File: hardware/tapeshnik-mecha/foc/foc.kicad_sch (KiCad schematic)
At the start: 32 parts, among them J1 Conn_01x03, J2 Conn_01x03, J3 Conn_01x02, J4 Conn_01x07, J5 Conn_01x03, J6 Conn_01x03, U1 STSPIN233, U2 INA181A1IDBVR, U3 MT6701, U4 INA181A1IDBVR, U5 RP2040-Zero, U6 MT6701, U7 STSPIN233, U8 INA181A1IDBVR, U9 INA181A1IDBVR

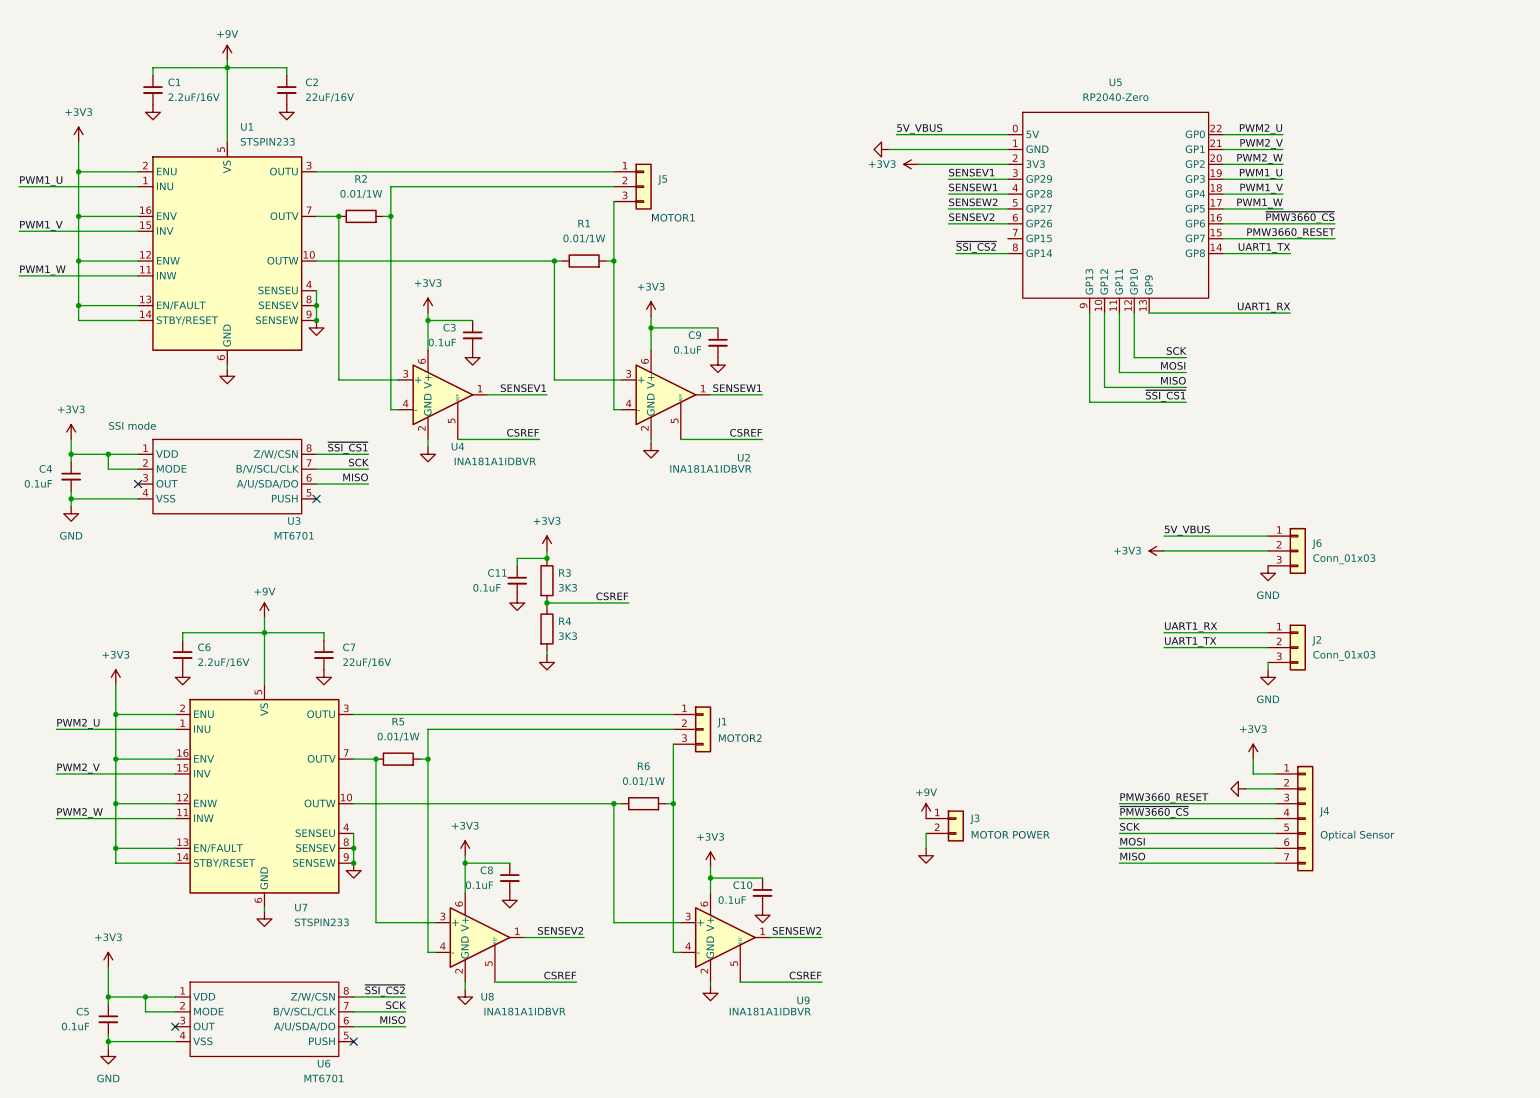
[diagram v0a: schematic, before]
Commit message: adding a lot of mecha-specific stuff
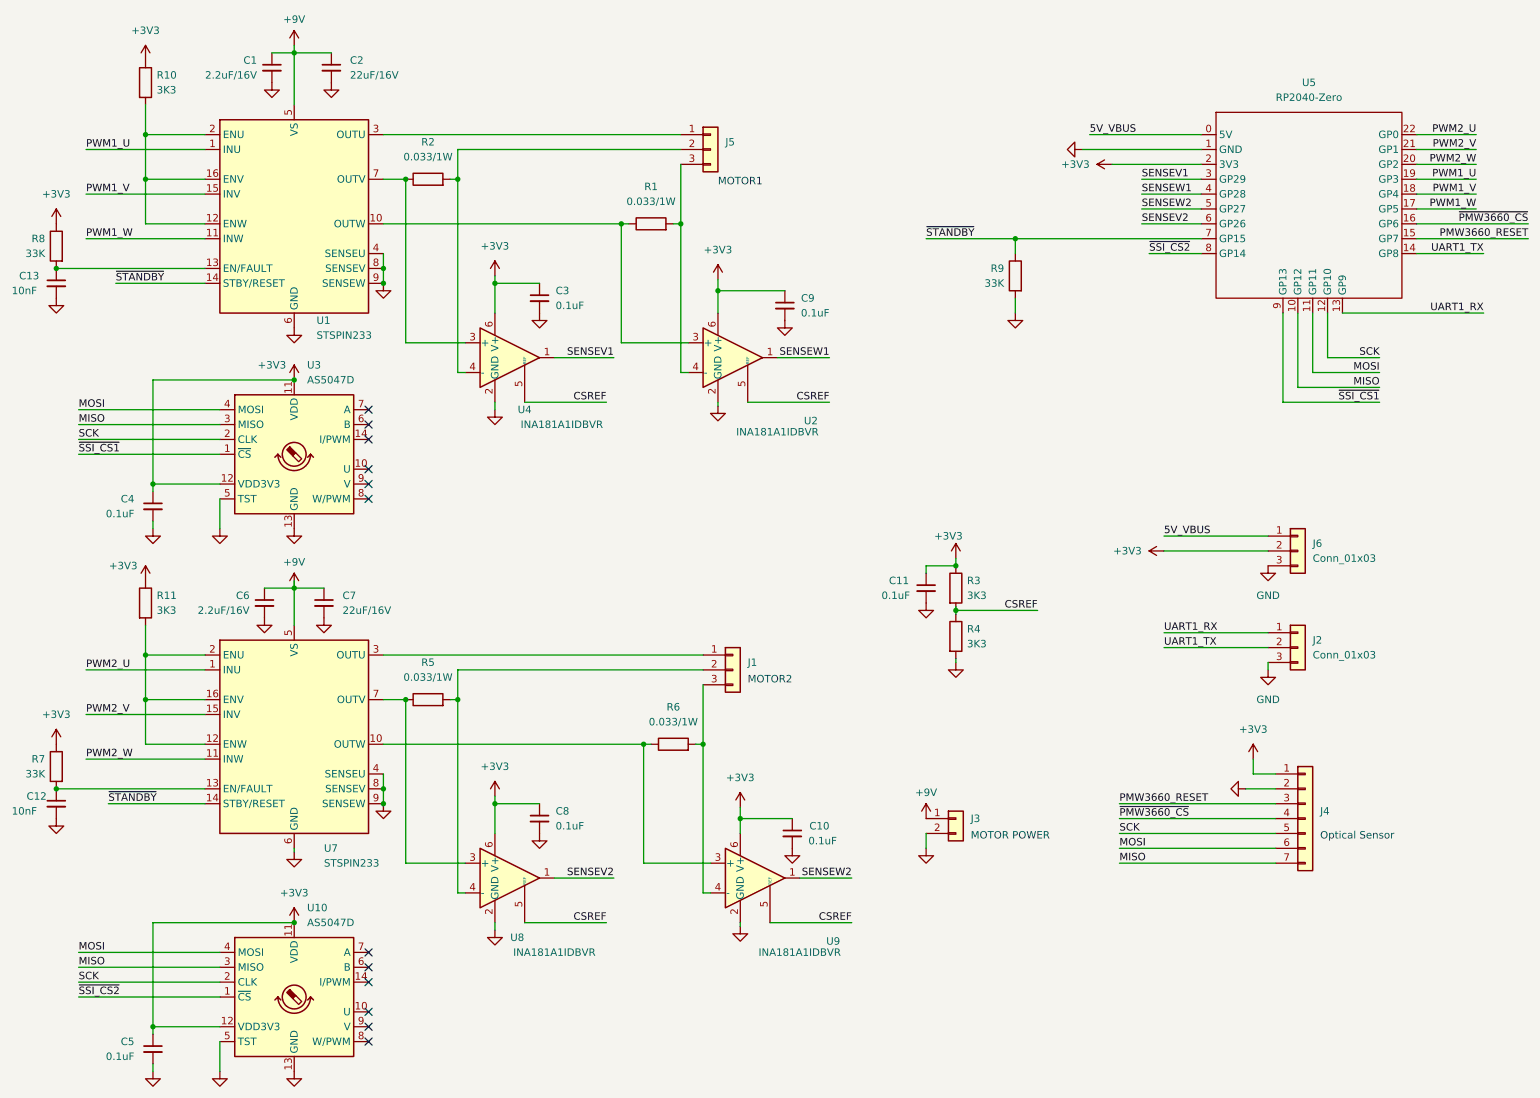
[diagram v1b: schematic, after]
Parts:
- removed U3, U6: MT6701, Package_SO:SOP-8_3.9x4.9mm_P1.27mm, symbol Magnetic_Encoder:MT6701
- added C12, C13: 10nF, Capacitor_SMD:C_0402_1005Metric, symbol Device:C_Small
- added R10, R11: 3K3, Resistor_SMD:R_0402_1005Metric, symbol Device:R
- added R7, R8: 33K, Resistor_SMD:R_0402_1005Metric, symbol Device:R
- added R9: 33K, Resistor_SMD:R_0603_1608Metric, symbol Device:R
- added U10, U3: AS5047D, Package_SO:TSSOP-14_4.4x5mm_P0.65mm, symbol Sensor_Magnetic:AS5047D
- C2, C7: footprint Capacitor_SMD:C_0603_1608Metric -> Capacitor_SMD:C_0805_2012Metric; LCSC (none) -> C45783
- R1, R2, R6: value 0.01/1W -> 0.033/1W; LCSC (none) -> C2934109
- R5: value 0.01/1W -> 0.033/1W; C55739 (none) -> C2934109
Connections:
- net +3V3: now also R10.1, R11.1, R7.1, R8.1, U10.11 (VDD), U10.12 (VDD3V3), U3.11 (VDD), U3.12 (VDD3V3); no longer U1.12 (ENW), U1.13 (EN/FAULT), U1.14 (STBY/RESET), U1.16 (ENV), U1.2 (ENU), U7.12 (ENW), U7.13 (EN/FAULT), U7.14 (STBY/RESET), U7.16 (ENV), U7.2 (ENU)
- net GND: now also C12.2, C13.2, R9.2, U10.13 (GND), U10.5 (TST), U3.13 (GND), U3.5 (TST)
- net MISO: now also U10.3 (MISO), U3.3 (MISO)
- net MOSI: now also U10.4 (MOSI), U3.4 (MOSI)
- net SCK: now also U10.2 (CLK), U3.2 (CLK)
- net ~{SSI_CS1}: now also U3.1 (~{CS})
- net ~{SSI_CS2}: now also U10.1 (~{CS})
- net ~{STANDBY}: now reaches U5.7 (GP15)
- net ~{STANDBY}: now also U1.14 (STBY/RESET), U7.14 (STBY/RESET), R9.1
- new net: R11.2, U7.12 (ENW), U7.16 (ENV), U7.2 (ENU)
- new net: C12.1, R7.2, U7.13 (EN/FAULT)
- new net: R10.2, U1.12 (ENW), U1.16 (ENV), U1.2 (ENU)
- new net: C13.1, R8.2, U1.13 (EN/FAULT)
- no-connect marks 4 -> 12
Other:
- note removed: "SSI mode"
- moved on the sheet: C1, C10, C11, C2, C3, C5, C6, C7, C8, C9, J1, J5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

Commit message: kicad file updates
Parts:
- R1, R2, R6: LCSC C2934109 -> C621267
- R5: C55739 C2934109 -> C621267
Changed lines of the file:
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@@
     (data
       iVBORw0KGgoAAAANSUhEUgAAA4QAAAPFCAIAAACyKLGlAAAAA3NCSVQICAjb4U/gAAAACXBIWXMA
-      AA7DAAAOwwHHb6hkAAAgAElEQVR4nOy9Wa8tyXXn918rIjJzD+fcsQYWSYmTqCbVUkNqG5IFuWW4
+      AA50AAAOdAFrJLPWAAAgAElEQVR4nOy9Wa8tyXXn918rIjJzD+fcsQYWSYmTqCbVUkNqG5IFuWW4
       bT/YgD+FH/wV/OoPYcCwAT/6wTD8aLeAlt3qbgEyWuqWRImiRBbnmu9whr13ZkastfwQmXn2Offe
       apZcdU8VuX642Hef3JmRc+Y/1hT0+PFjOI7jOI7jOM5twLe9AY7jOI7jOM4vLi5GHcdxHMdxnFvD
@@
       (effects (font (size 1.27 1.27)) hide)
     )
-    (property "LCSC" "C2934109" (at 127 138.43 90)
+    (property "LCSC" "C621267" (at 127 138.43 90)
       (effects (font (size 1.27 1.27)) hide)
     )
@@
       (effects (font (size 1.27 1.27)) hide)
     )
-    (property "LCSC" "C2934109" (at 123.19 49.53 90)
+    (property "LCSC" "C621267" (at 123.19 49.53 90)
       (effects (font (size 1.27 1.27)) hide)
     )
@@
       (effects (font (size 1.27 1.27)) hide)
     )
-    (property "C55739" "C2934109" (at 85.09 130.81 90)
+    (property "C55739" "C621267" (at 85.09 130.81 90)
       (effects (font (size 1.27 1.27)) hide)
     )
@@
       (effects (font (size 1.27 1.27)) hide)
     )
-    (property "LCSC" "C2934109" (at 85.09 41.91 90)
+    (property "LCSC" "C621267" (at 85.09 41.91 90)
       (effects (font (size 1.27 1.27)) hide)
     )
